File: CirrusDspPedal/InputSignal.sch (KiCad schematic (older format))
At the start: 24 parts, among them J1 MonoJack2Switch, U1 CS5343, U2 74AHC1G126, U8 TPS60400, U9 OPA197IDBV

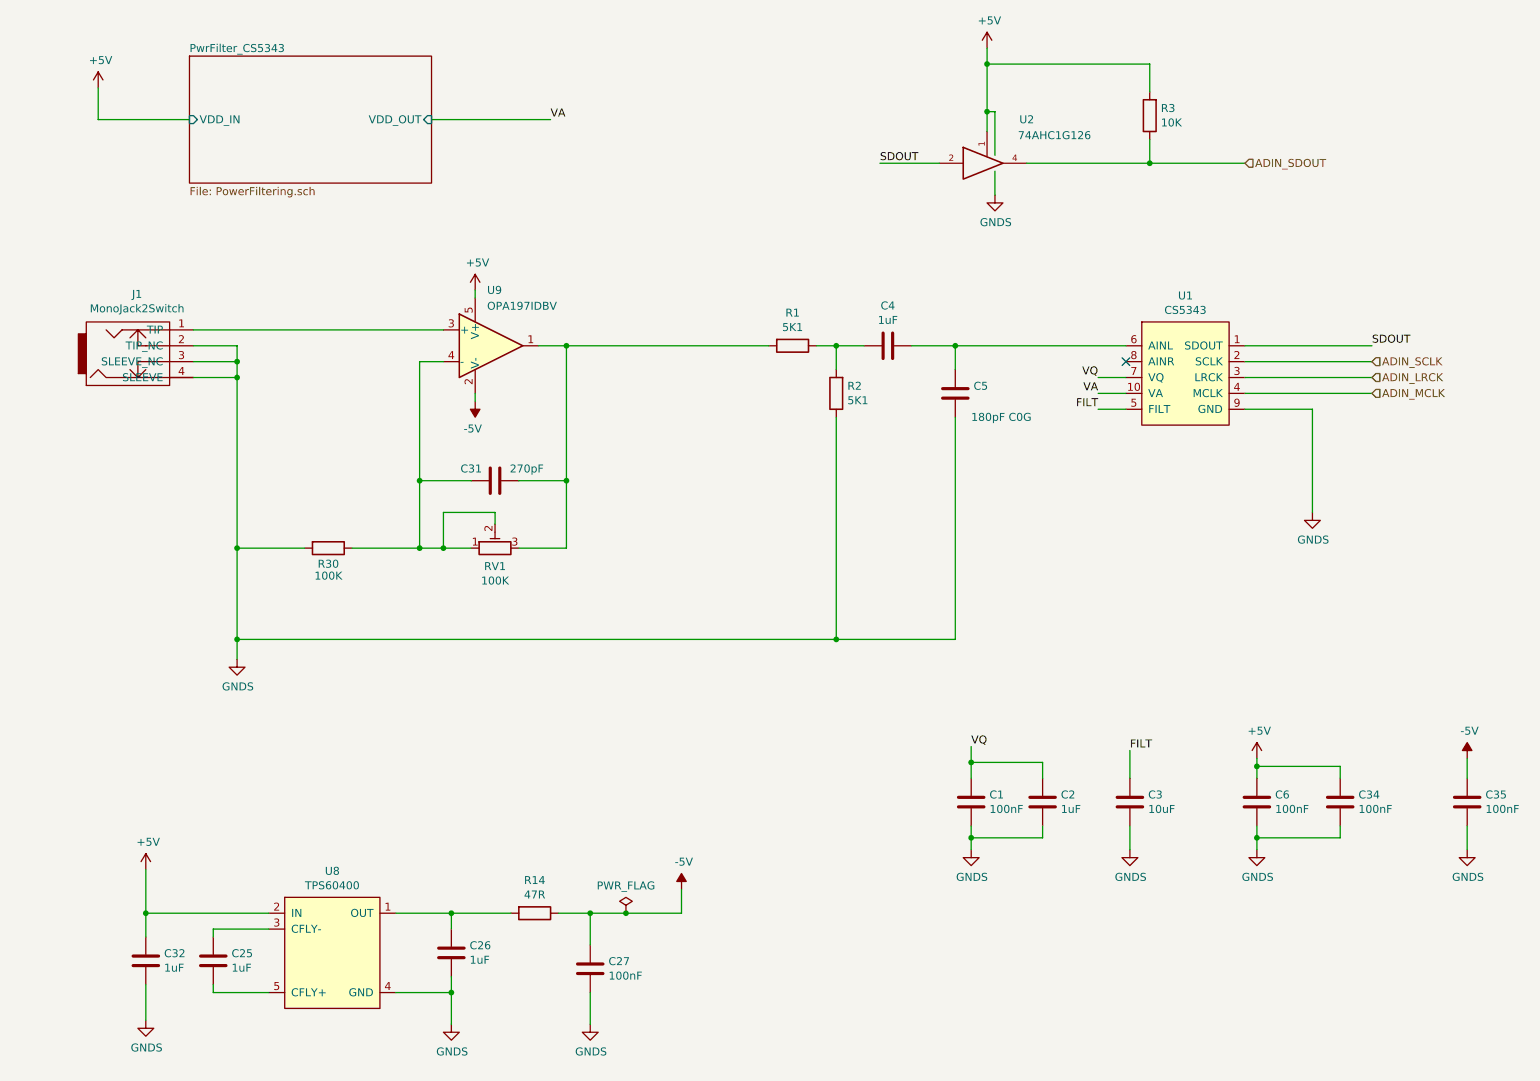
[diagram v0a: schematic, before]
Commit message: final revb layout
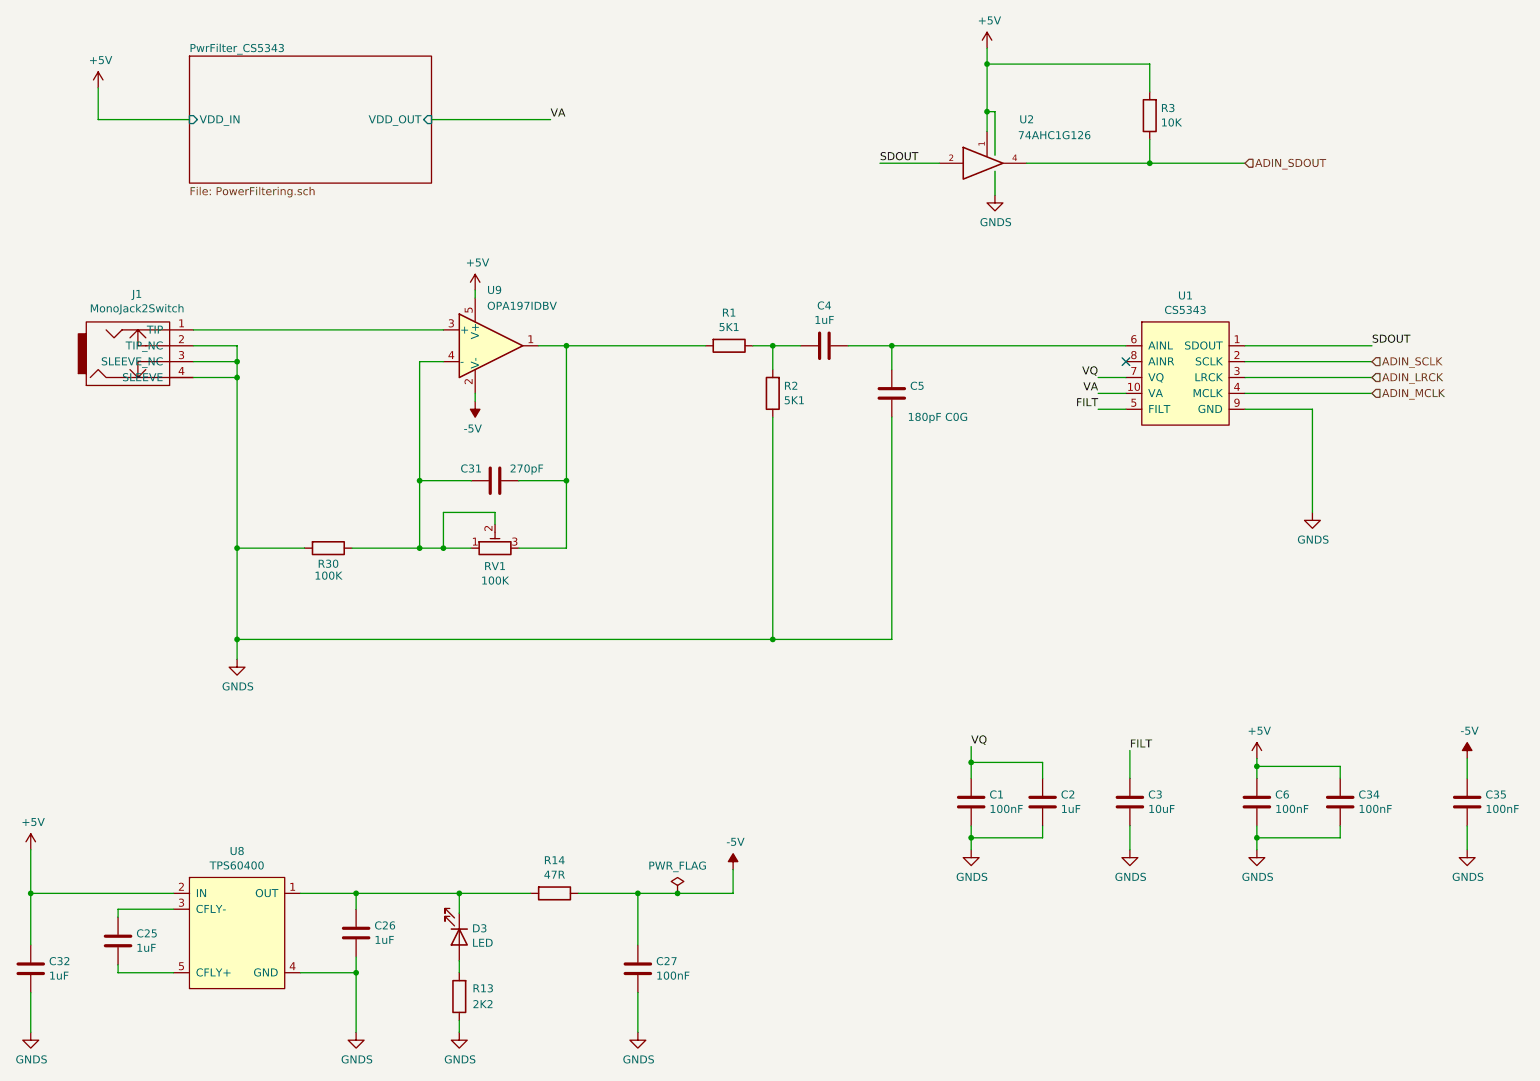
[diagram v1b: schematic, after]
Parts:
- added D3: LED, LED_SMD:LED_0805_2012Metric_Pad1.15x1.40mm_HandSolder, symbol Device:LED
- added R13: 2K2, Resistor_SMD:R_0805_2012Metric_Pad1.20x1.40mm_HandSolder, symbol Device:R
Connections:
- net GND: now also R13.1
- net at C26.1, R14.2, U8.1 (OUT): now also D3.1 (K)
- new net: D3.2 (A), R13.2
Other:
- moved on the sheet: C25, C26, C27, C32, C4, C5, R1, R14, R2, U8
